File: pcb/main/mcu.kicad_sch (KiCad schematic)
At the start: 31 parts, among them J1 UART, J2 JTAG, J3 JTAG SRC, J4 26 pin IDC, J5 Conn_01x06, SW1 Boot, SW2 Reset, U1 74LVC1G17, U2 74LVC1G17, U3 ESP32-S3-WROOM-1

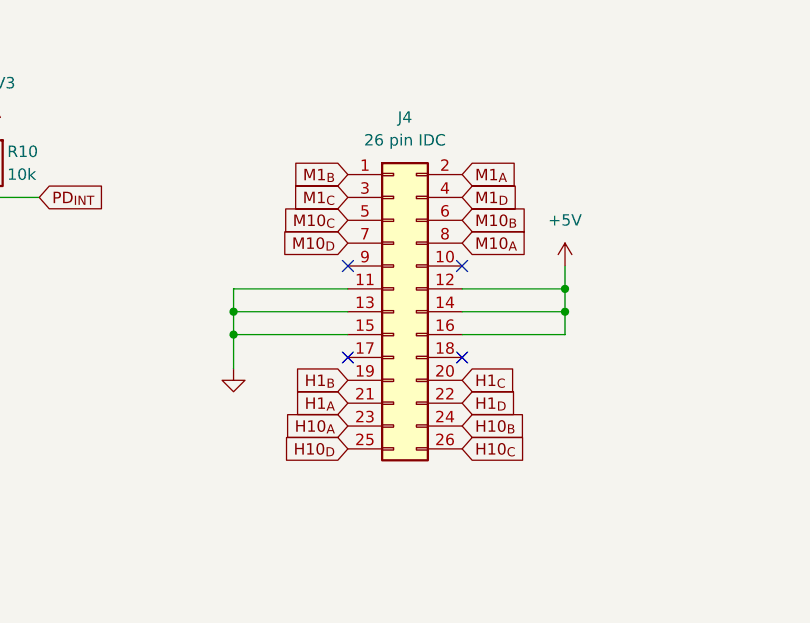
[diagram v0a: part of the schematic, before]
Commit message: Clock Face Rev C
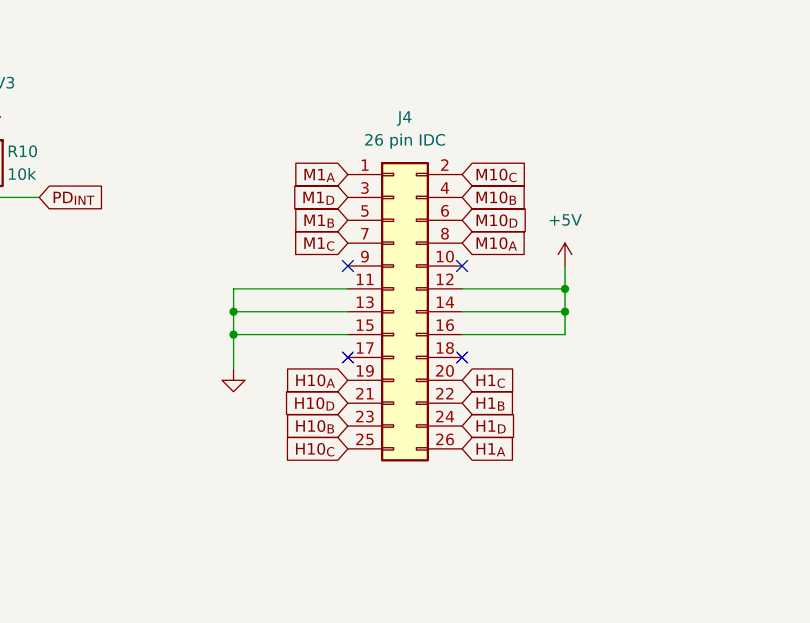
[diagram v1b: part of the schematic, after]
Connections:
- net H10_{A}: now also J4.19 (Pin_19); no longer J4.23 (Pin_23)
- net H10_{B}: now also J4.23 (Pin_23); no longer J4.24 (Pin_24)
- net H10_{C}: now also J4.25 (Pin_25); no longer J4.26 (Pin_26)
- net H10_{D}: now also J4.21 (Pin_21); no longer J4.25 (Pin_25)
- net H1_{A}: now also J4.26 (Pin_26); no longer J4.21 (Pin_21)
- net H1_{B}: now also J4.22 (Pin_22); no longer J4.19 (Pin_19)
- net H1_{D}: now also J4.24 (Pin_24); no longer J4.22 (Pin_22)
- net M10_{B}: now also J4.4 (Pin_4); no longer J4.6 (Pin_6)
- net M10_{C}: now also J4.2 (Pin_2); no longer J4.5 (Pin_5)
- net M10_{D}: now also J4.6 (Pin_6); no longer J4.7 (Pin_7)
- net M1_{A}: now also J4.1 (Pin_1); no longer J4.2 (Pin_2)
- net M1_{B}: now also J4.5 (Pin_5); no longer J4.1 (Pin_1)
- net M1_{C}: now also J4.7 (Pin_7); no longer J4.3 (Pin_3)
- net M1_{D}: now also J4.3 (Pin_3); no longer J4.4 (Pin_4)

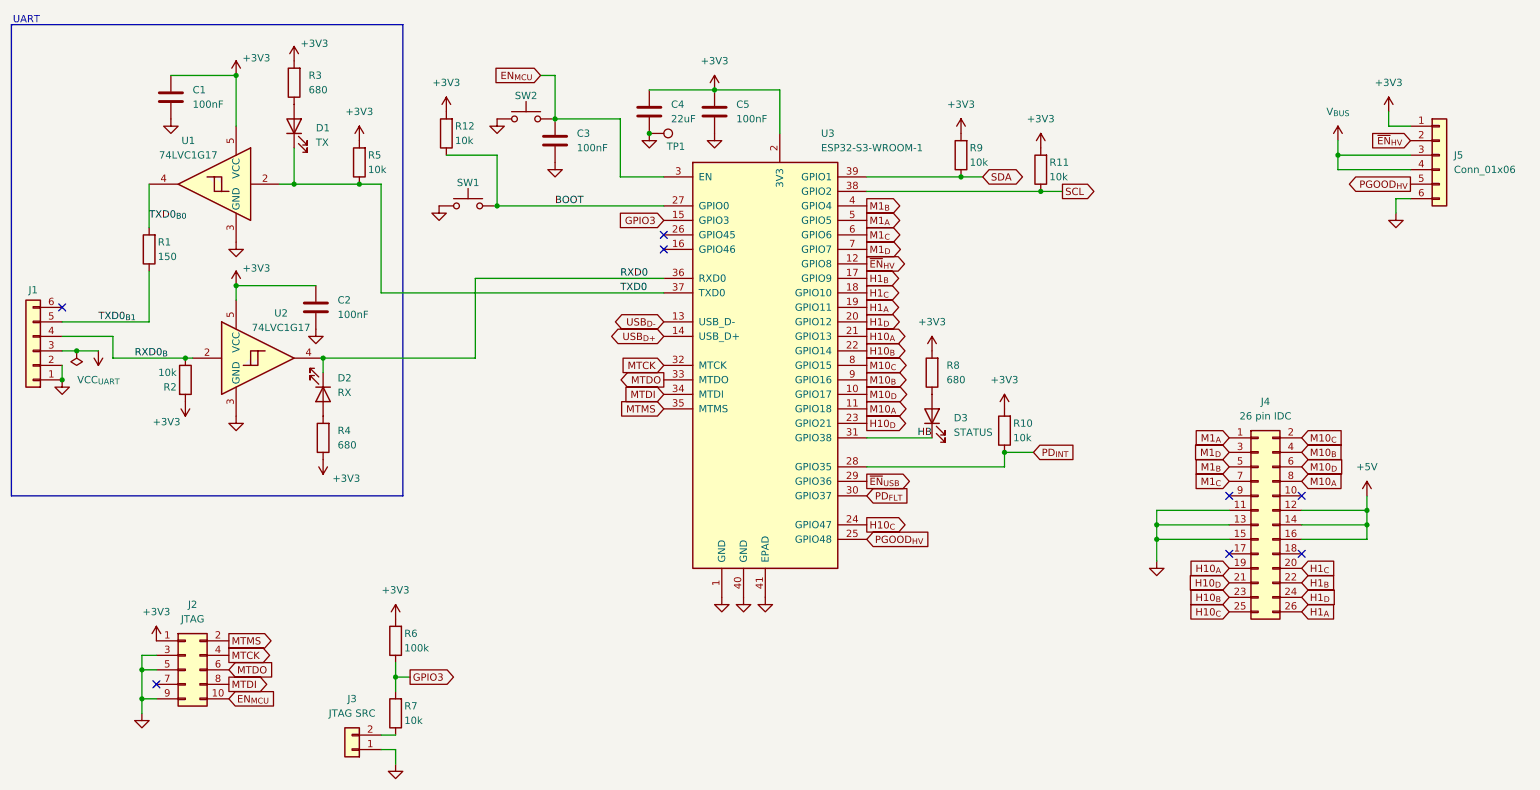
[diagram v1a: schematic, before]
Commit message: Main board Rev C
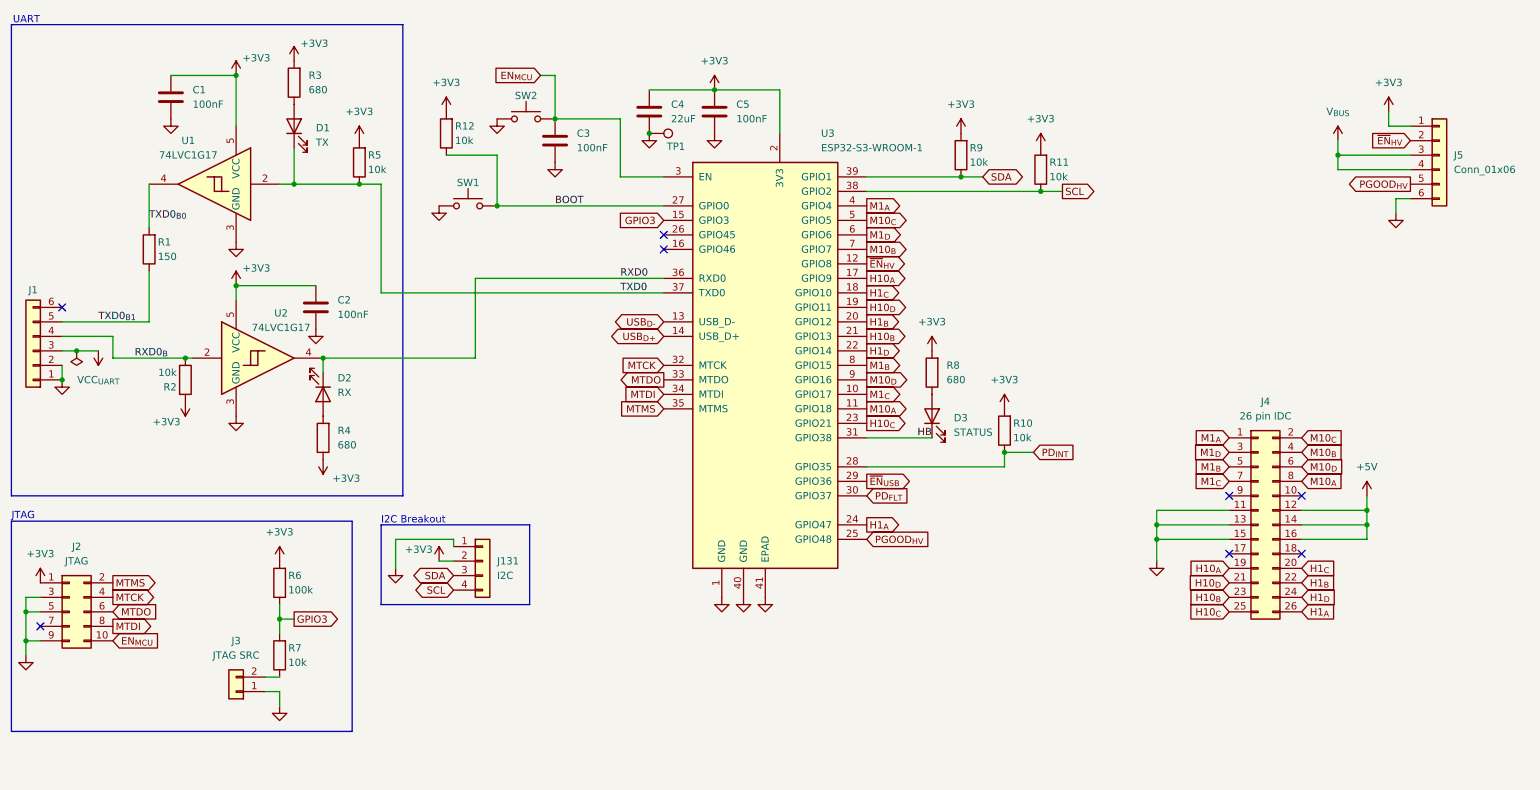
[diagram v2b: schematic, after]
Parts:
- added J131: I2C, Connector_PinHeader_2.54mm:PinHeader_1x04_P2.54mm_Vertical, symbol Connector_Generic:Conn_01x04
- J3: footprint Connector_PinHeader_2.54mm:PinHeader_1x02_P2.54mm_Vertical -> Connector_PinHeader_1.27mm:PinHeader_1x02_P1.27mm_Vertical; MFG Part No (none) -> M50-3530242; Note (none) -> Close with M50-1900005 or equivelent
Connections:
- net +3V3: now also J131.2 (Pin_2)
- net GND: now also J131.1 (Pin_1)
- net H10_{A}: now also U3.17 (GPIO9); no longer U3.21 (GPIO13)
- net H10_{B}: now also U3.21 (GPIO13); no longer U3.22 (GPIO14)
- net H10_{C}: now also U3.23 (GPIO21); no longer U3.24 (GPIO47)
- net H10_{D}: now also U3.19 (GPIO11); no longer U3.23 (GPIO21)
- net H1_{A}: now also U3.24 (GPIO47); no longer U3.19 (GPIO11)
- net H1_{B}: now also U3.20 (GPIO12); no longer U3.17 (GPIO9)
- net H1_{D}: now also U3.22 (GPIO14); no longer U3.20 (GPIO12)
- net M10_{B}: now also U3.7 (GPIO7); no longer U3.9 (GPIO16)
- net M10_{C}: now also U3.5 (GPIO5); no longer U3.8 (GPIO15)
- net M10_{D}: now also U3.9 (GPIO16); no longer U3.10 (GPIO17)
- net M1_{A}: now also U3.4 (GPIO4); no longer U3.5 (GPIO5)
- net M1_{B}: now also U3.8 (GPIO15); no longer U3.4 (GPIO4)
- net M1_{C}: now also U3.10 (GPIO17); no longer U3.6 (GPIO6)
- net M1_{D}: now also U3.6 (GPIO6); no longer U3.7 (GPIO7)
- net SCL: now also J131.4 (Pin_4)
- net SDA: now also J131.3 (Pin_3)
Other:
- note added: "I2C Breakout"
- note added: "JTAG"
- moved on the sheet: J2, J3, R6, R7
